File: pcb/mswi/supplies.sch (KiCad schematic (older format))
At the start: 11 parts, among them Q601 si2308cds, U601 LM7805

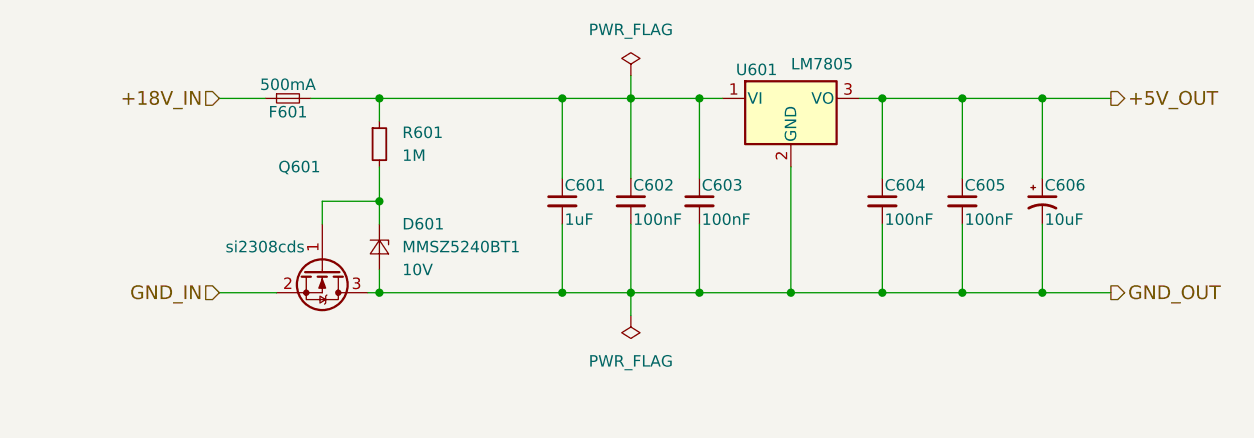
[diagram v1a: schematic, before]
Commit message: TVS added
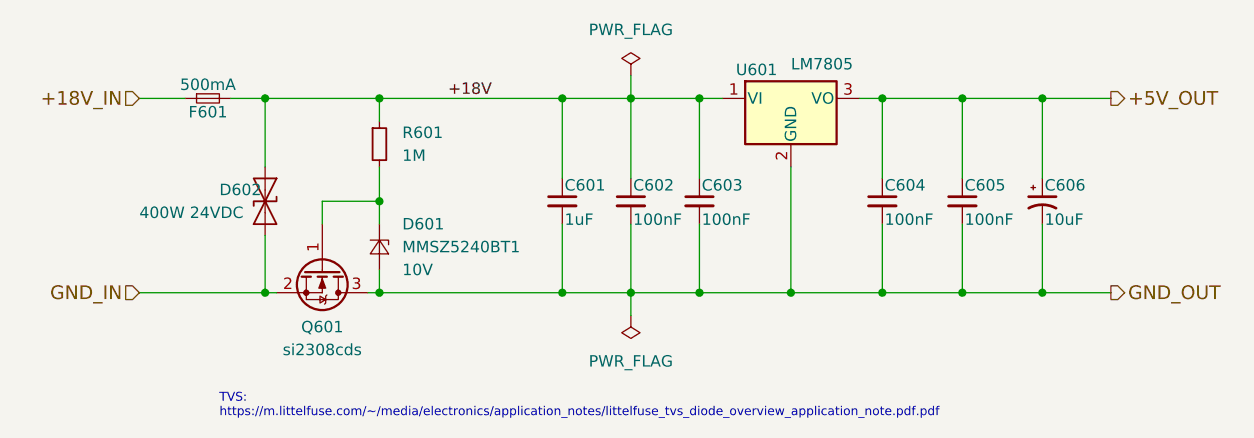
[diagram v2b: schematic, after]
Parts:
- added D602: 400W 24VDC, Diode_SMD:D_SMA, symbol Device:D_TVS
- F601: Model (none) -> 0ZCJ0050AF2E; Mouser (none) -> https://br.mouser.com/ProductDetail/Bel-Fuse/0ZCJ0050AF2E?q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
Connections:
- net GND_IN: now also D602.2 (A2)
- net +18V: now reaches C601.1, C602.1, C603.1, F601.2, R601.1, U601.1 (VI)
- net +18V: now also D602.1 (A1)
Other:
- note added: "TVS:\nhttps://m.littelfuse.com/~~/media/electronics/application_notes/littelfuse_tvs_diode_overview_application_note.pdf.pdf"
- moved on the sheet: F601
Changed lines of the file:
@@
 	1    0    0    -1
 $EndComp
-Text HLabel 3400 4800 0    60   Input ~ 0
+Text HLabel 3050 4800 0    60   Input ~ 0
 GND_IN
 Text HLabel 7300 3950 2    60   Output ~ 0
@@
 	1    0    0    -1
 $EndComp
-Text HLabel 3400 3950 0    60   Input ~ 0
+Text HLabel 3050 3950 0    60   Input ~ 0
 +18V_IN
 $Comp
@@
 L Device:Fuse_Small F601
 U 1 1 5AB12173
-P 3700 3950
+P 3350 3950
 AR Path="/5AACFFEF/5AB12173" Ref="F601"  Part="1"
 AR Path="/5DDD6AD9/5AB12173" Ref="F?"  Part="1"
 AR Path="/5DDDDD89/5AB12173" Ref="F?"  Part="1"
-F 0 "F601" H 3700 3890 50  0000 C CNN
-F 1 "500mA" H 3700 4010 50  0000 C CNN
-F 2 "Fuse:Fuse_1206_3216Metric_Pad1.42x1.75mm_HandSolder" H 3700 3950 50  0001 C CNN
-F 3 "https://www.mouser.com/datasheet/2/643/0ZCJ_Nov2016-1132002.pdf" H 3700 3950 50  0001 C CNN
-	1    3700 3950
+F 0 "F601" H 3350 3890 50  0000 C CNN
+F 1 "500mA" H 3350 4010 50  0000 C CNN
+F 2 "Fuse:Fuse_1206_3216Metric_Pad1.42x1.75mm_HandSolder" H 3350 3950 50  0001 C CNN
+F 3 "https://www.mouser.com/datasheet/2/643/0ZCJ_Nov2016-1132002.pdf" H 3350 3950 50  0001 C CNN
+F 4 "https://br.mouser.com/ProductDetail/Bel-Fuse/0ZCJ0050AF2E?qs=%2Fha2pyFadugaoNql5zaJPtCzxaRCuZne0%252BGltuyizoH09DOBIA3TDQ%3D%3D" H 3350 3950 50  0001 C CNN "Mouser"
+F 5 "0ZCJ0050AF2E" H 3350 3950 50  0001 C CNN "Model"
+	1    3350 3950
 	1    0    0    -1
 $EndComp
@@
 	4900 3950 4900 4300
 Wire Wire Line
-	3800 3950 4100 3950
+	3450 3950 3600 3950
 Wire Wire Line
 	4900 3950 5200 3950
@@
 	7000 4800 7300 4800
 Wire Wire Line
-	3400 3950 3600 3950
+	3050 3950 3250 3950
 Wire Wire Line
 	4050 4800 4100 4800
@@
 AR Path="/5DDD6AD9/5D9E3E7E" Ref="Q?"  Part="1"
 AR Path="/5DDDDD89/5D9E3E7E" Ref="Q?"  Part="1"
-F 0 "Q601" V 3400 4600 50  0000 C CNN
-F 1 "si2308cds" V 3750 4450 50  0000 C CNN
+F 0 "Q601" V 4100 4700 50  0000 C CNN
+F 1 "si2308cds" V 4200 4700 50  0000 C CNN
 F 2 "Package_TO_SOT_SMD:SOT-23" H 4050 4800 50  0001 C CNN
 F 3 "~" H 3850 4700 50  0001 C CNN
@@
 Connection ~ 4100 3950
 Wire Wire Line
-	4100 3950 4900 3950
-Wire Wire Line
 	4100 4700 4100 4800
 Wire Wire Line
@@
 	4100 4400 4100 4500
 Wire Wire Line
-	3400 4800 3650 4800
+	3050 4800 3600 4800
 $Comp
 L Device:C_Small C603
@@
 Wire Wire Line
 	5200 3850 5200 3950
+Wire Wire Line
+	4100 3950 4900 3950
+Text Label 4400 3950 0    50   ~ 0
++18V
+$Comp
+L Device:D_TVS D602
+U 1 1 5DD19DD4
+P 3600 4400
+F 0 "D602" V 3550 4600 50  0000 R CNN
+F 1 "400W 24VDC" V 3650 4950 50  0000 R CNN
+F 2 "Diode_SMD:D_SMA" H 3600 4400 50  0001 C CNN
+F 3 "https://www.mouser.com/datasheet/2/445/824501241-952945.pdf" H 3600 4400 50  0001 C CNN
+F 4 "https://br.mouser.com/ProductDetail/Wurth-Elektronik/824501241?qs=%2Fha2pyFadujZKBgF5S1ldkLPpipTn8KXCRHX4IsQDUlguH4XSGuxlw%3D%3D" V 3600 4400 50  0001 C CNN "Mouser"
+	1    3600 4400
+	0    -1   1    0
+$EndComp
+Wire Wire Line
+	3600 4250 3600 3950
+Connection ~ 3600 3950
+Wire Wire Line
+	3600 3950 4100 3950
+Wire Wire Line
+	3600 4550 3600 4800
+Connection ~ 3600 4800
+Wire Wire Line
+	3600 4800 3650 4800
+Text Notes 3400 5350 0    39   ~ 0
+TVS:\nhttps://m.littelfuse.com/~~/media/electronics/application_notes/littelfuse_tvs_diode_overview_application_note.pdf.pdf
 $EndSCHEMATC
